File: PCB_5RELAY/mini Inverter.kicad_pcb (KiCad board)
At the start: 2 copper layers, 102.7 x 70 mm, 50 parts, among them IC1 ULN2003, SW1 Nút Nhấn 6x6mm Cao 5.5mm 2 Ch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, SW2 Nút Nhấn 6x6mm Cao 5.5mm 2 Ch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, SW3 Nút Nhấn 6x6mm Cao 5.5mm 2 Ch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, SW4 Nút Nhấn 6x6mm Cao 5.5mm 2 Ch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, SW5 Nút Nhấn 6x6mm Cao 5.5mm 2 Ch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, SW6 Nút Nhấn 6x6mm Cao 5.5mm 2 Ch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, U1 HLK-10M-12 (10W), U2 L7805, U3 AMS1117, U4 ESP32-WROOM-32E

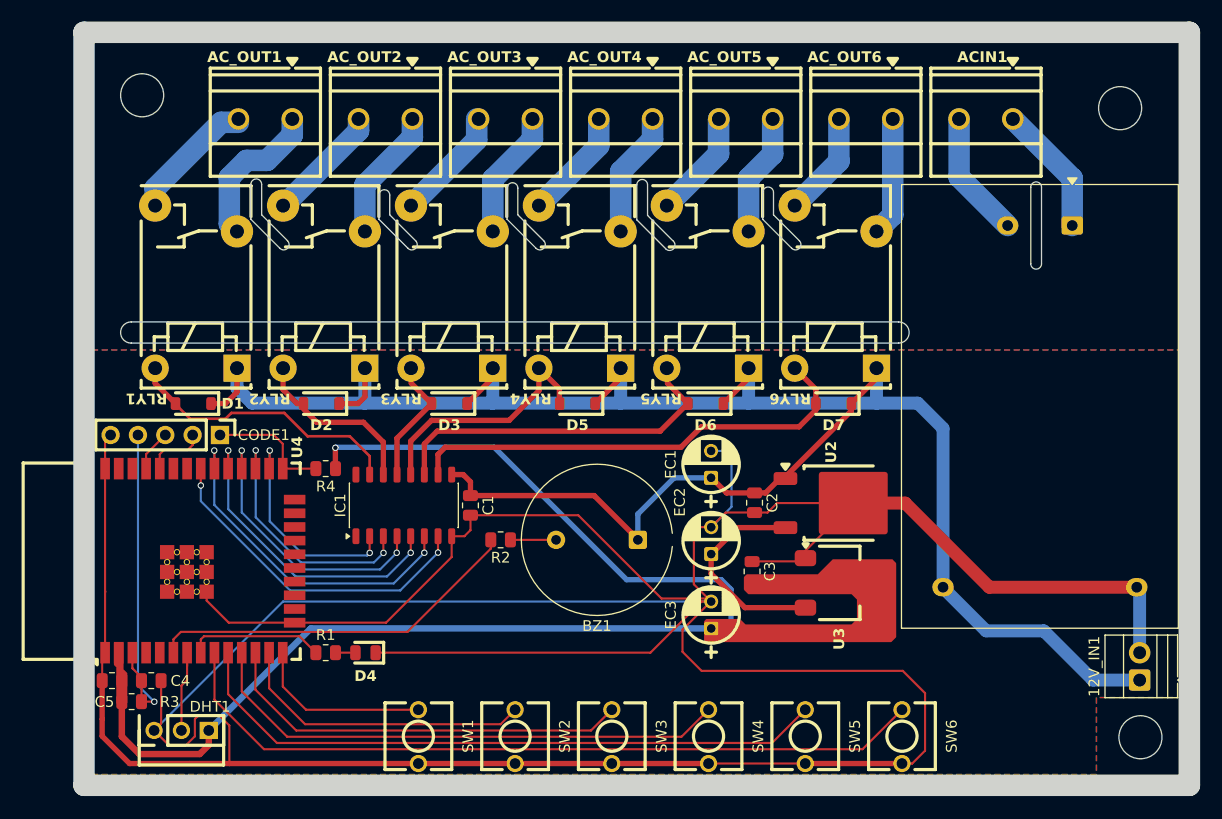
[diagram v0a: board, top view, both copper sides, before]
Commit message: 916102026"
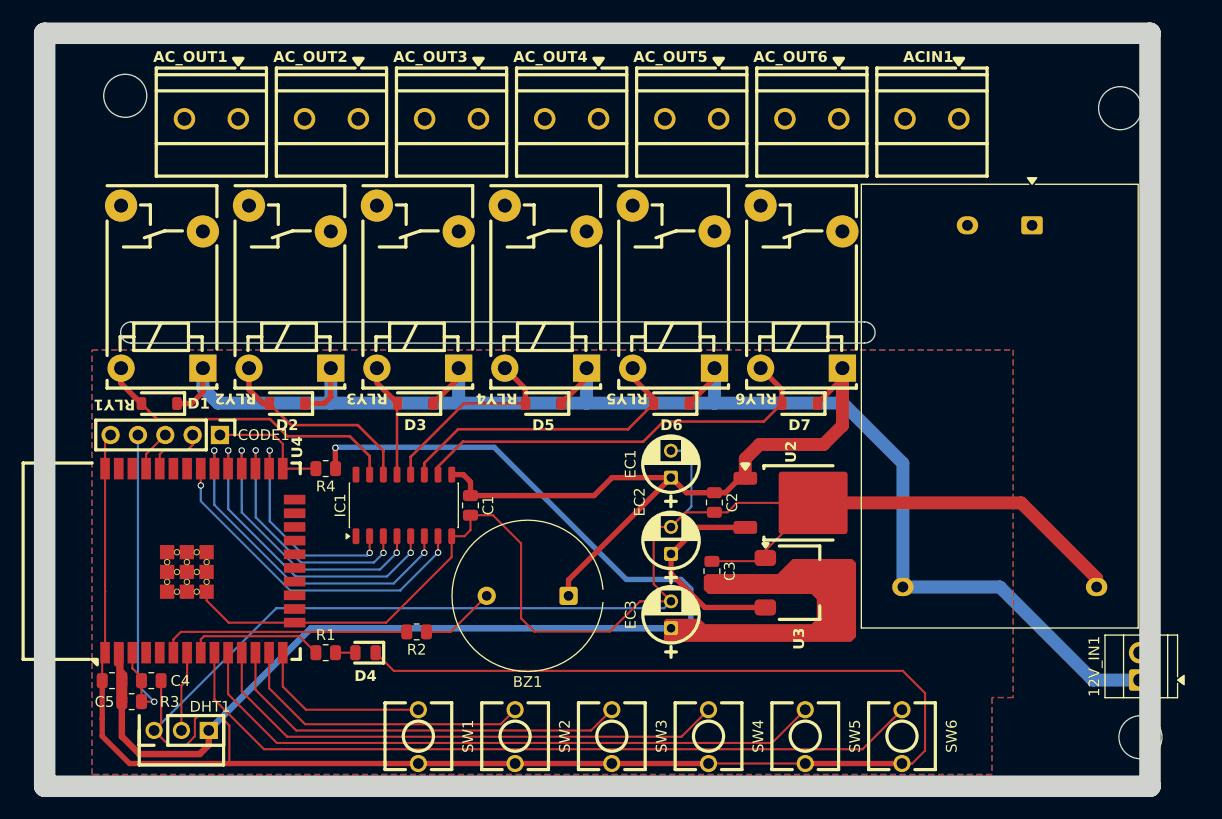
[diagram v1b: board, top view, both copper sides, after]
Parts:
- moved R2 11.6 mm to (126.8, 125.5)
- moved BZ1 8.28 mm to (140.9, 122.2)
- moved AC_OUT1 5.02 mm to (107.7, 77.9)
- moved AC_OUT2 5.02 mm to (118.8, 77.9)
- moved ACIN1 5.02 mm to (174.6, 77.9)
- moved AC_OUT3 5.02 mm to (130.0, 77.9)
- moved AC_OUT4 5.02 mm to (141.2, 77.9)
- moved AC_OUT5 5.02 mm to (152.3, 77.9)
- moved AC_OUT6 5.02 mm to (163.5, 77.9)
- moved EC2 3.73 mm to (150.4, 117.1)
- moved EC3 3.73 mm to (150.4, 124.0)
- moved U1 3.73 mm to (183.9, 87.8)
- moved U3 3.73 mm to (162.3, 121.0)
- moved C2 3.73 mm to (154.4, 113.5)
- moved C3 3.73 mm to (154.2, 119.9)
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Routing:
- net GND: track 387.7 -> 371.2 mm
- net +12V: track 198.1 -> 213.8 mm
- net /ACOUT12: track 14.3 -> 0.00 mm
- net /ACOUT22: track 12.3 -> 0.00 mm
- net /ACL: track 12.2 -> 0.00 mm
- net /ACOUT32: track 12.0 -> 0.00 mm
- net /ACOUT11: track 11.9 -> 0.00 mm
- net /ACN: track 11.8 -> 0.00 mm
- net /BUZZ: track 35.0 -> 23.3 mm
- net /ACOUT42: track 11.7 -> 0.00 mm
- net /ACOUT52: track 11.4 -> 0.00 mm
- net /ACOUT62: track 11.1 -> 0.00 mm
- net /ACOUT21: track 10.9 -> 0.00 mm
- net /ACOUT31: track 10.6 -> 0.00 mm
- net /ACOUT41: track 10.4 -> 0.00 mm
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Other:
- board size 102.7 x 70 mm -> 102.7 x 69.9 mm
